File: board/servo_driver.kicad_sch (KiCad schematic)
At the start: 23 parts, among them U5 PCA9685PW

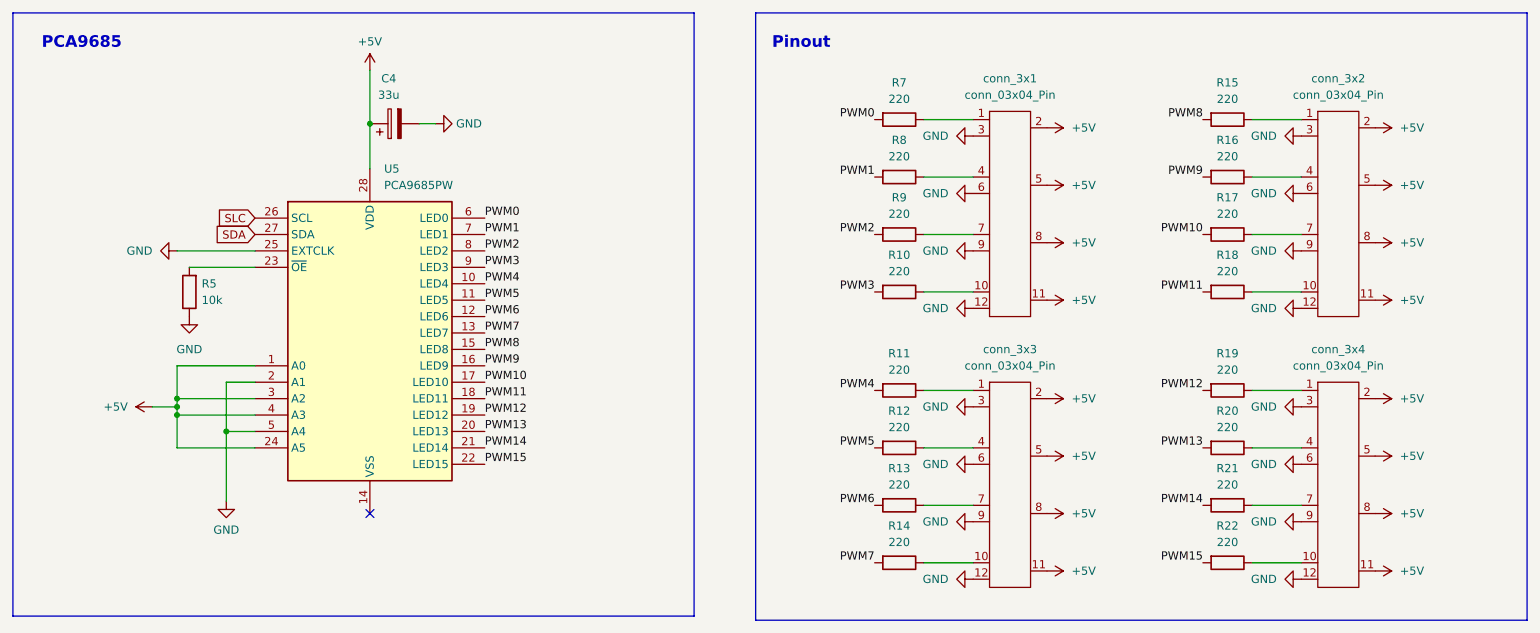
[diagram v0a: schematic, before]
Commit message: First version of PCB finished
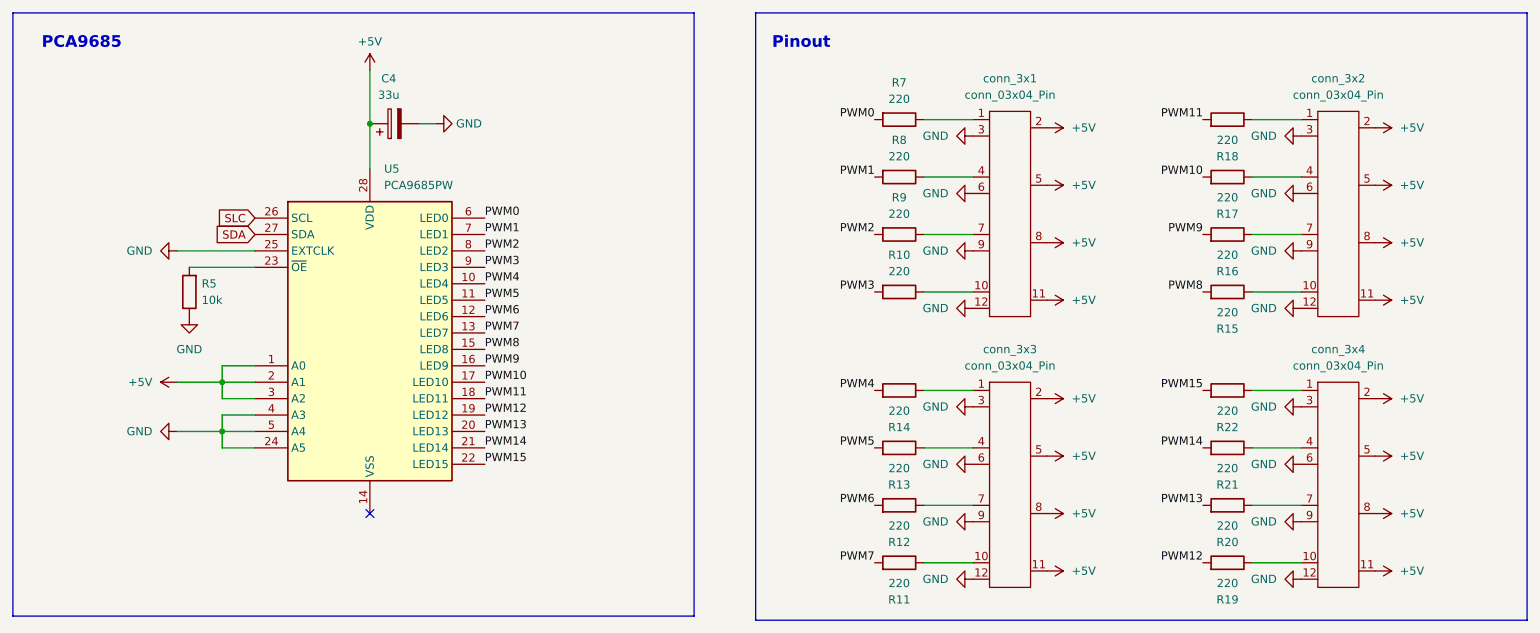
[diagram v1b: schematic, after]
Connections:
- net +5V: now also U5.2 (A1); no longer U5.24 (A5), U5.4 (A3)
- net GND: now also U5.24 (A5), U5.4 (A3); no longer U5.2 (A1)
- net PWM4: now also R14.2; no longer R11.2
- net PWM5: now also R13.2; no longer R12.2
- net PWM6: now also R12.2; no longer R13.2
- net PWM7: now also R11.2; no longer R14.2
- net at R11.1: now also conn_3x3.10; no longer conn_3x3.1
- net at conn_3x2.1: now also R18.1; no longer R15.1
- net at conn_3x2.10: now also R15.1; no longer R18.1
- net at conn_3x2.4: now also R17.1; no longer R16.1
- net at conn_3x2.7: now also R16.1; no longer R17.1
- net at R13.1: now also conn_3x3.4; no longer conn_3x3.7
- net at R21.1: now also conn_3x4.4; no longer conn_3x4.7
- net at conn_3x4.1: now also R22.1; no longer R19.1
- net at conn_3x4.10: now also R19.1; no longer R22.1
- net at R20.1: now also conn_3x4.7; no longer conn_3x4.4
- net at R14.1: now also conn_3x3.1; no longer conn_3x3.10
- net at R12.1: now also conn_3x3.7; no longer conn_3x3.4
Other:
- moved on the sheet: R11, R12, R13, R14, R15, R16, R17, R18, R19, R20, R21, R22
